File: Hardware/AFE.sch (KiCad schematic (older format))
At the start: 40 parts, among them U801 4069.HEF4069UBTT,118, U802 MCP47CXBX2

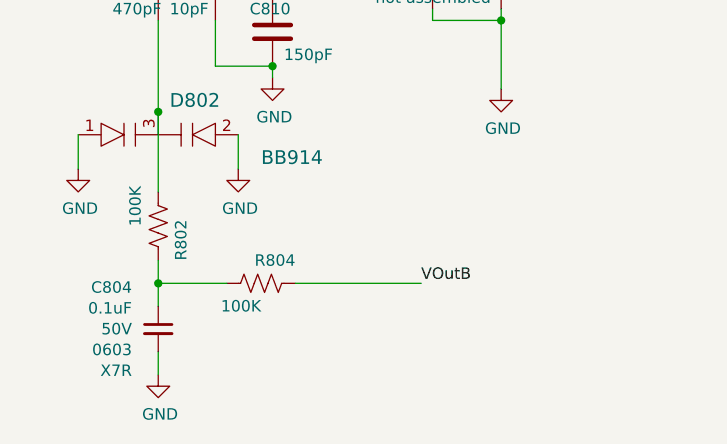
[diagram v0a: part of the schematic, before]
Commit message: Placements mostly done.
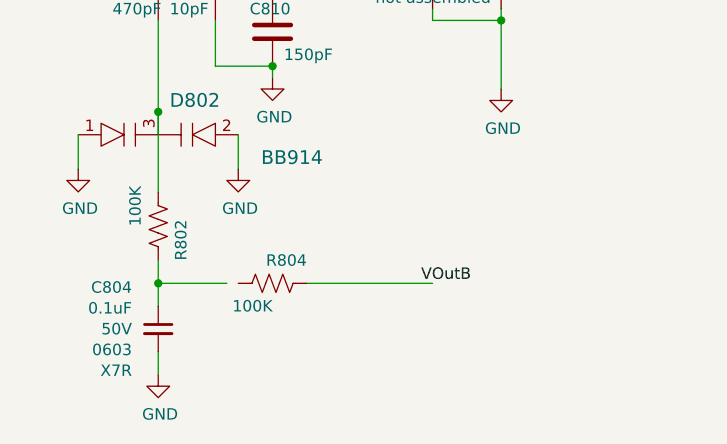
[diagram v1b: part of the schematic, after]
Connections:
- net at C804.1, R802.2: no longer R804.1
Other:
- moved on the sheet: R804
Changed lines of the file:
@@
 L Device:R_US R?
 U 1 1 6165DF0B
-P 1500 7000
+P 1550 7000
 AR Path="/611E335F/6165DF0B" Ref="R?"  Part="1"
 AR Path="/612429E8/6165DF0B" Ref="R804"  Part="1"
-F 0 "R804" V 1600 6850 50  0000 L CNN
-F 1 "100K" V 1400 7000 50  0000 L CNN
-F 2 "Resistor_SMD:R_0603_1608Metric" V 1430 7000 50  0001 C CNN
-F 3 "~" H 1500 7000 50  0001 C CNN
-F 4 "0603" H 1500 7000 50  0001 C CNN "Pkg"
-F 5 "ESR03EZPJ104" H 1500 7000 50  0001 C CNN "MPN"
-F 6 "RHM100KDCT-ND" H 1500 7000 50  0001 C CNN "DPN"
-	1    1500 7000
+F 0 "R804" V 1650 6850 50  0000 L CNN
+F 1 "100K" V 1450 7000 50  0000 L CNN
+F 2 "Resistor_SMD:R_0603_1608Metric" V 1480 7000 50  0001 C CNN
+F 3 "~" H 1550 7000 50  0001 C CNN
+F 4 "0603" H 1550 7000 50  0001 C CNN "Pkg"
+F 5 "ESR03EZPJ104" H 1550 7000 50  0001 C CNN "MPN"
+F 6 "RHM100KDCT-ND" H 1550 7000 50  0001 C CNN "DPN"
+	1    1550 7000
 	0    -1   -1   0
 $EndComp
 Wire Wire Line
-	1650 7000 2200 7000
+	1700 7000 2250 7000
 Wire Wire Line
 	1050 7000 1350 7000
